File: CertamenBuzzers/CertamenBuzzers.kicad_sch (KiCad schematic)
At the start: 53 parts, among them J1 USB_C_Receptacle_USB2.0_14P, J10 RJ45, J11 RJ45, J12 RJ45, J13 RJ45, J2 RJ45, J3 RJ45, J4 RJ45, J5 RJ45, J6 RJ45, J7 RJ45, J8 RJ45, J9 RJ45, SW1 BOOT, SW2 RST, U1 RP2040, U2 NCP1117-3.3_SOT223, U3 TVS1400DRV, U4 W25Q32JVZP, Y1 12MHz

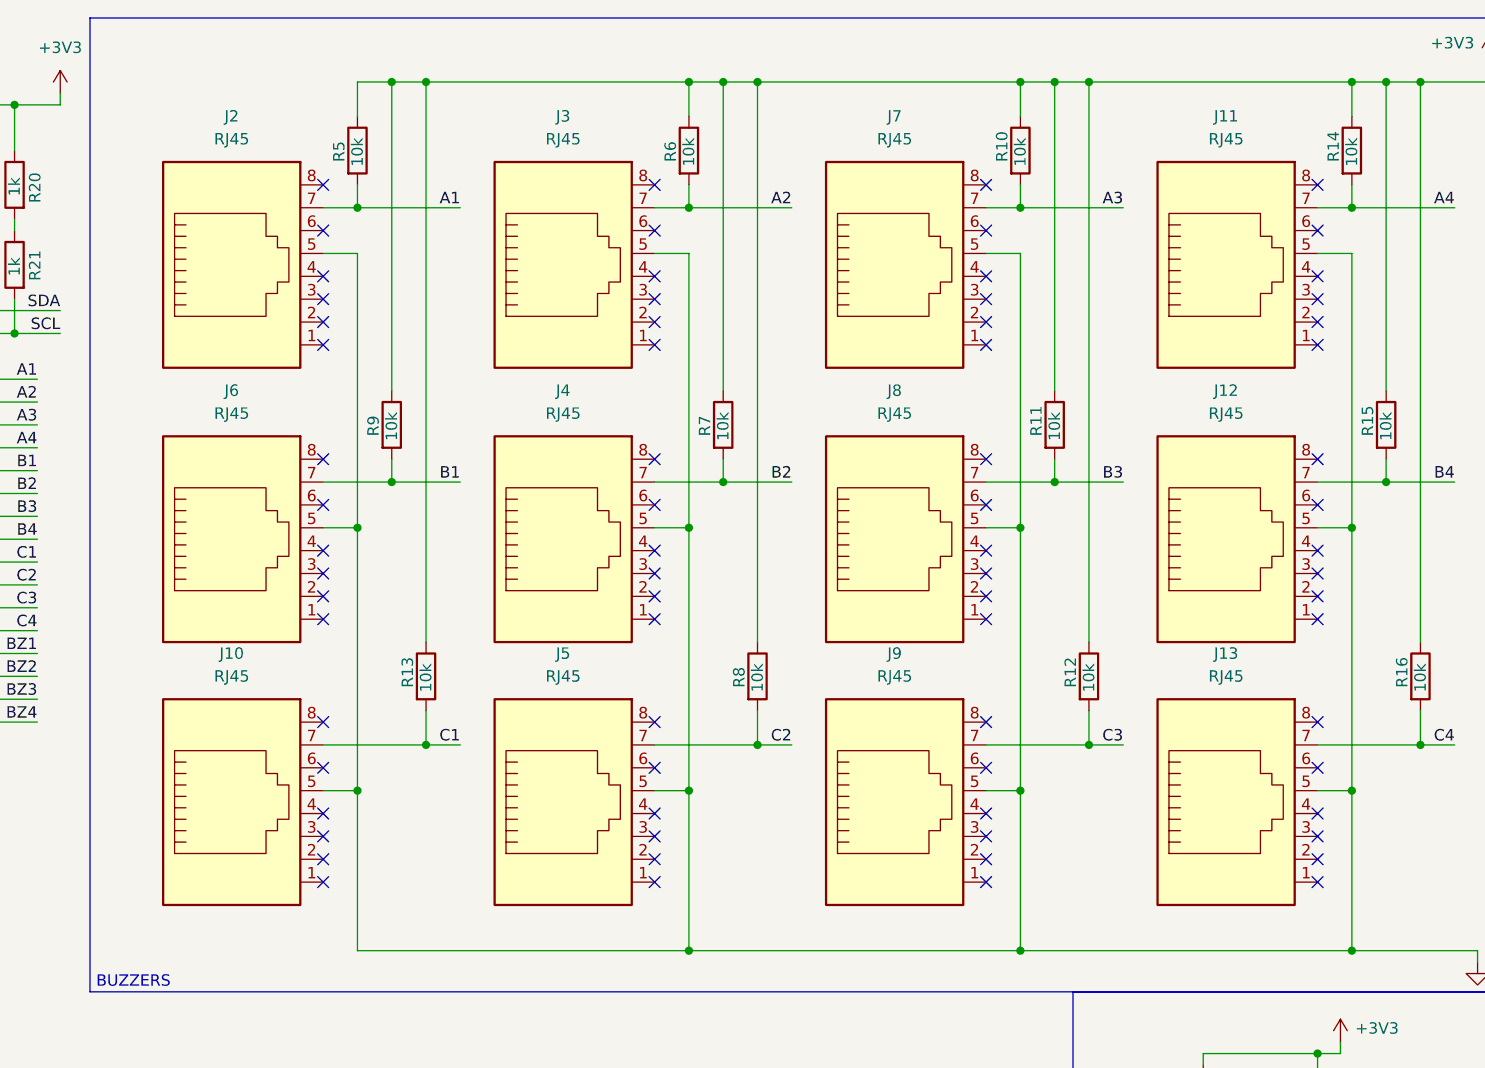
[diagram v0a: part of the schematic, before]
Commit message: scheamtic done + cost optimized some more
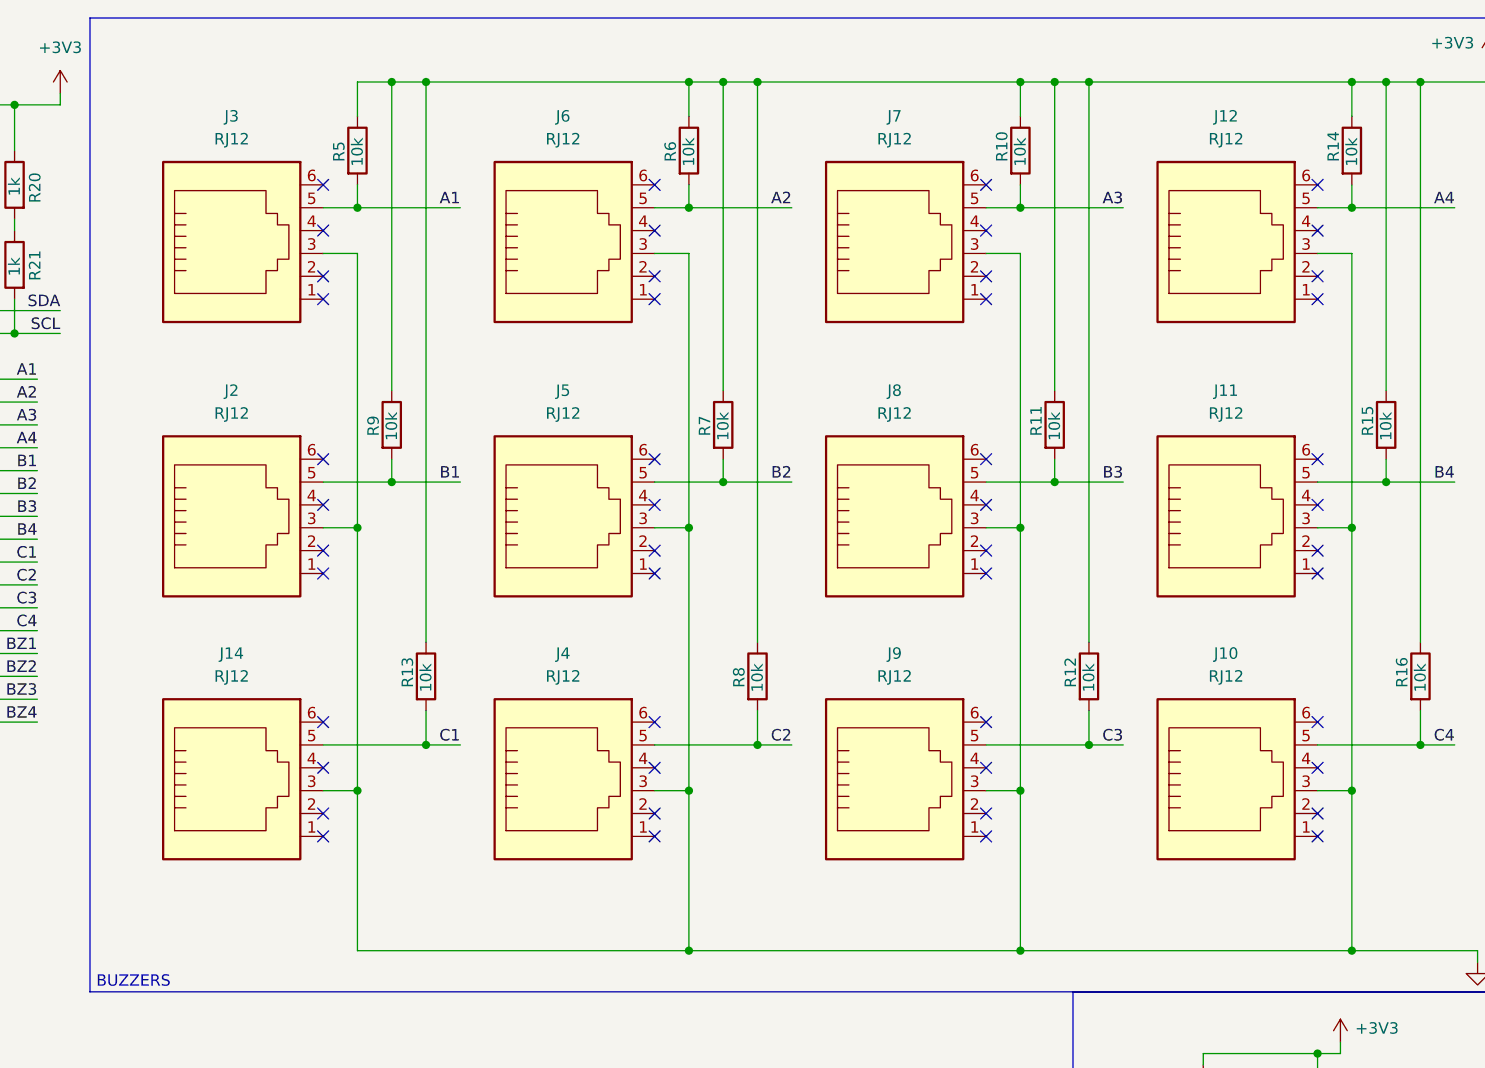
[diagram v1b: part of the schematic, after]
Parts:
- removed J10, J11, J12, J13, J2, J3, J4, J5, J6, J7, J8, J9: RJ45, Buzzers:ADAMTECH_MTJ-88ARX1-FSM-LG, symbol Connector:RJ45
- added J10, J11, J12, J14, J2, J3, J4, J5, J6, J7, J8, J9: RJ12, Buzzers:ADAMTECH_MTJ-88ARX1-FSM-LG, symbol Connector:RJ12
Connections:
- net A1: now also J3.5
- net A2: now also J6.5
- net A3: now also J7.5
- net A4: now also J12.5
- net B1: now also J2.5
- net B2: now also J5.5
- net B3: now also J8.5
- net B4: now also J11.5
- net C1: now also J14.5
- net C2: now also J4.5
- net C3: now also J9.5
- net C4: now also J10.5
- net GND: now also J10.3, J11.3, J12.3, J14.3, J2.3, J3.3, J4.3, J5.3, J6.3, J7.3, J8.3, J9.3
- no-connect marks 86 -> 62
